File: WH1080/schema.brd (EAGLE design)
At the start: 78.4 x 97.8 mm, 18 parts

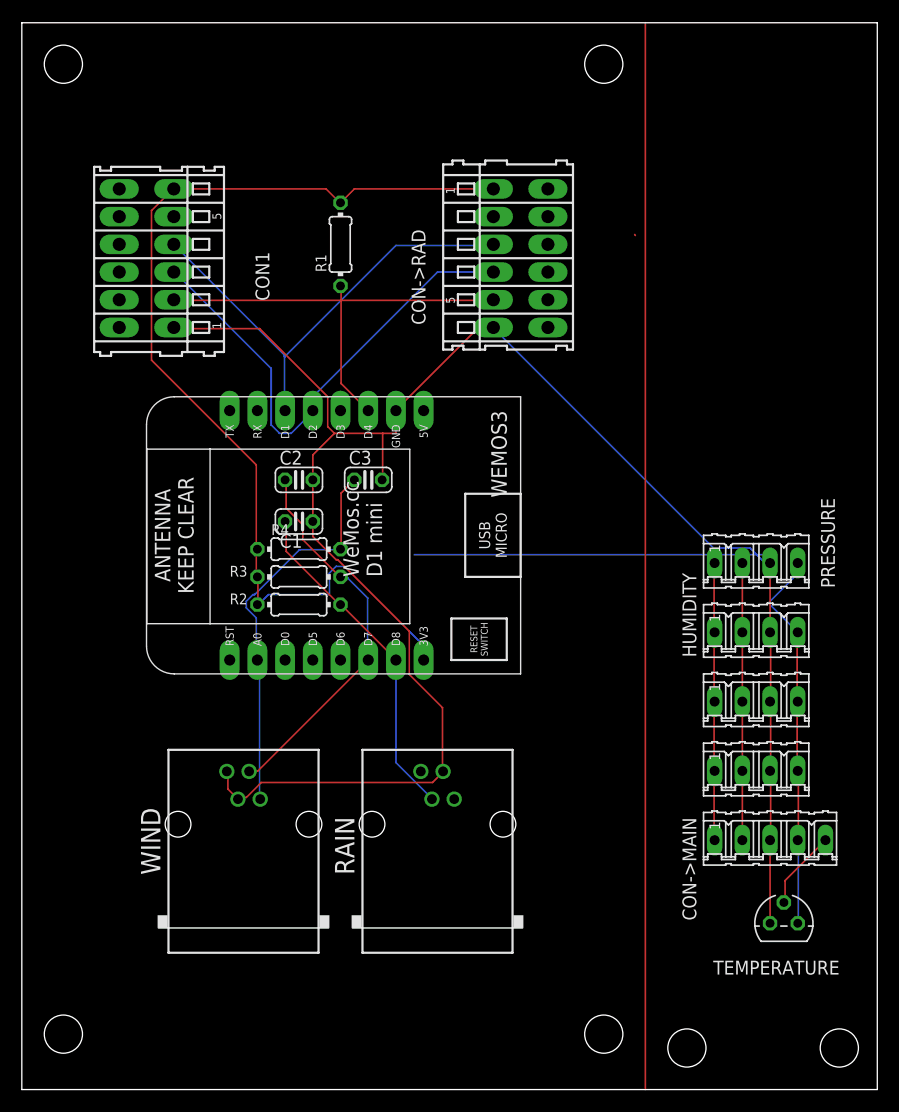
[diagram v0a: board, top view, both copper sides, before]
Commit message: +
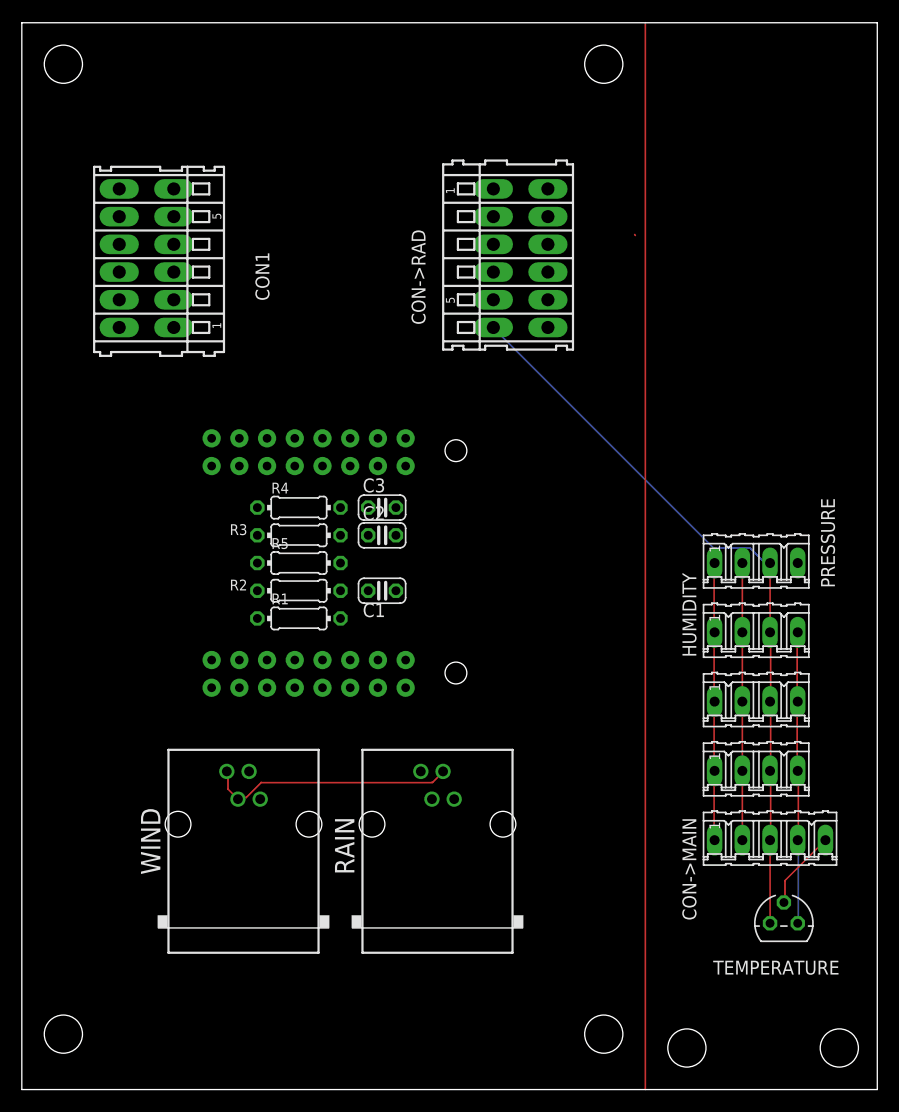
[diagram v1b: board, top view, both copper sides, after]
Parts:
- removed WEMOS3: (no value), esp8266modules:WEMOS-D1-MINI
- added R5: 4k7, rcl:0204/7
- added U$1: WEMOS_S2_MINI, Wemos_Boards:S2_MINI
- moved R1 34.5 mm to (25.4, 43.2), turned to 0 degrees
- moved C1 9.92 mm to (33.0, 45.7)
- moved C2 9.16 mm to (33.0, 50.8)
- moved R4 3.81 mm to (25.4, 53.3)
- moved R3 3.81 mm to (25.4, 50.8)
- moved C3 2.84 mm to (33.0, 53.3)
- moved R2 1.27 mm to (25.4, 45.7)
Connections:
- removed net +5V: WEMOS3.5V
- removed net N$3: CON->RAD.B5, CON1.B2, R1.1, WEMOS3.D4
- removed net N$5: CON->RAD.B3, CON1.B4, WEMOS3.D1
- removed net N$7: CON->RAD.B4, CON1.B3, WEMOS3.D2
- new net GND2: U$1.P22
- new net N$10: CON->MAIN.1, HUMIDITY.1, PRESSURE.1, SL3.1, SL4.1
- new net N$11: CON->MAIN.2, HUMIDITY.2, PRESSURE.2, SL3.2, SL4.2
- new net N$12: U$1.P0
- new net N$13: CON1.B1, R1.2, U$1.P1
- new net N$14: CON->RAD.B1, U$1.P5
- new net N$15: U$1.P9
- new net N$16: U$1.P10
- new net N$17: U$1.P11
- new net VBUS: U$1.P7
- net +3V3: now also CON->RAD.B2, CON1.B2, R1.1, R5.1, U$1.P8; no longer CON->RAD.B1, CON1.B6, R1.2, WEMOS3.3V3
- net GND: now also CON->RAD.B3, CON1.B3, U$1.P6; no longer CON->RAD.B6, CON1.B1, WEMOS3.GND
- net N$1: now also U$1.P13; no longer WEMOS3.D8
- net N$2: now also U$1.P12; no longer WEMOS3.A0
- net N$4: now also U$1.P14; no longer WEMOS3.D7
- net N$9: now also R5.2
- net SCL: now also CON->RAD.B5, CON1.B5, U$1.P2; no longer CON->MAIN.2, HUMIDITY.2, PRESSURE.2, SL3.2, SL4.2
- net SDA: now also CON->RAD.B4, CON1.B4, U$1.P3; no longer CON->MAIN.1, HUMIDITY.1, PRESSURE.1, SL3.1, SL4.1
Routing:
- net +3V3: track 163.7 -> 28.0 mm
- net GND: track 171.8 -> 90.0 mm
- net N$7: track 45.4 -> 0.00 mm
- net N$5: track 42.9 -> 0.00 mm
- net N$3: track 41.8 -> 0.00 mm
- net N$2: track 36.1 -> 0.00 mm
- net N$4: track 35.3 -> 0.00 mm
- net N$1: track 31.2 -> 0.00 mm
- net N$10: track 0.00 -> 25.6 mm
- net SDA: track 25.6 -> 0.14 mm
- net SCL: track 25.4 -> 0.00 mm
- net N$11: track 0.00 -> 25.4 mm
